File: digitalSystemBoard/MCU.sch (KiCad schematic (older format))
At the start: 33 parts, among them J1 USB-B, SW9 ButtonFirst, U10 74HC165, U11 74HC595, U6 ATmega32U4-AU, U7 ICSP, U8 74HC165, U9 74HC595, Y0 16MHz

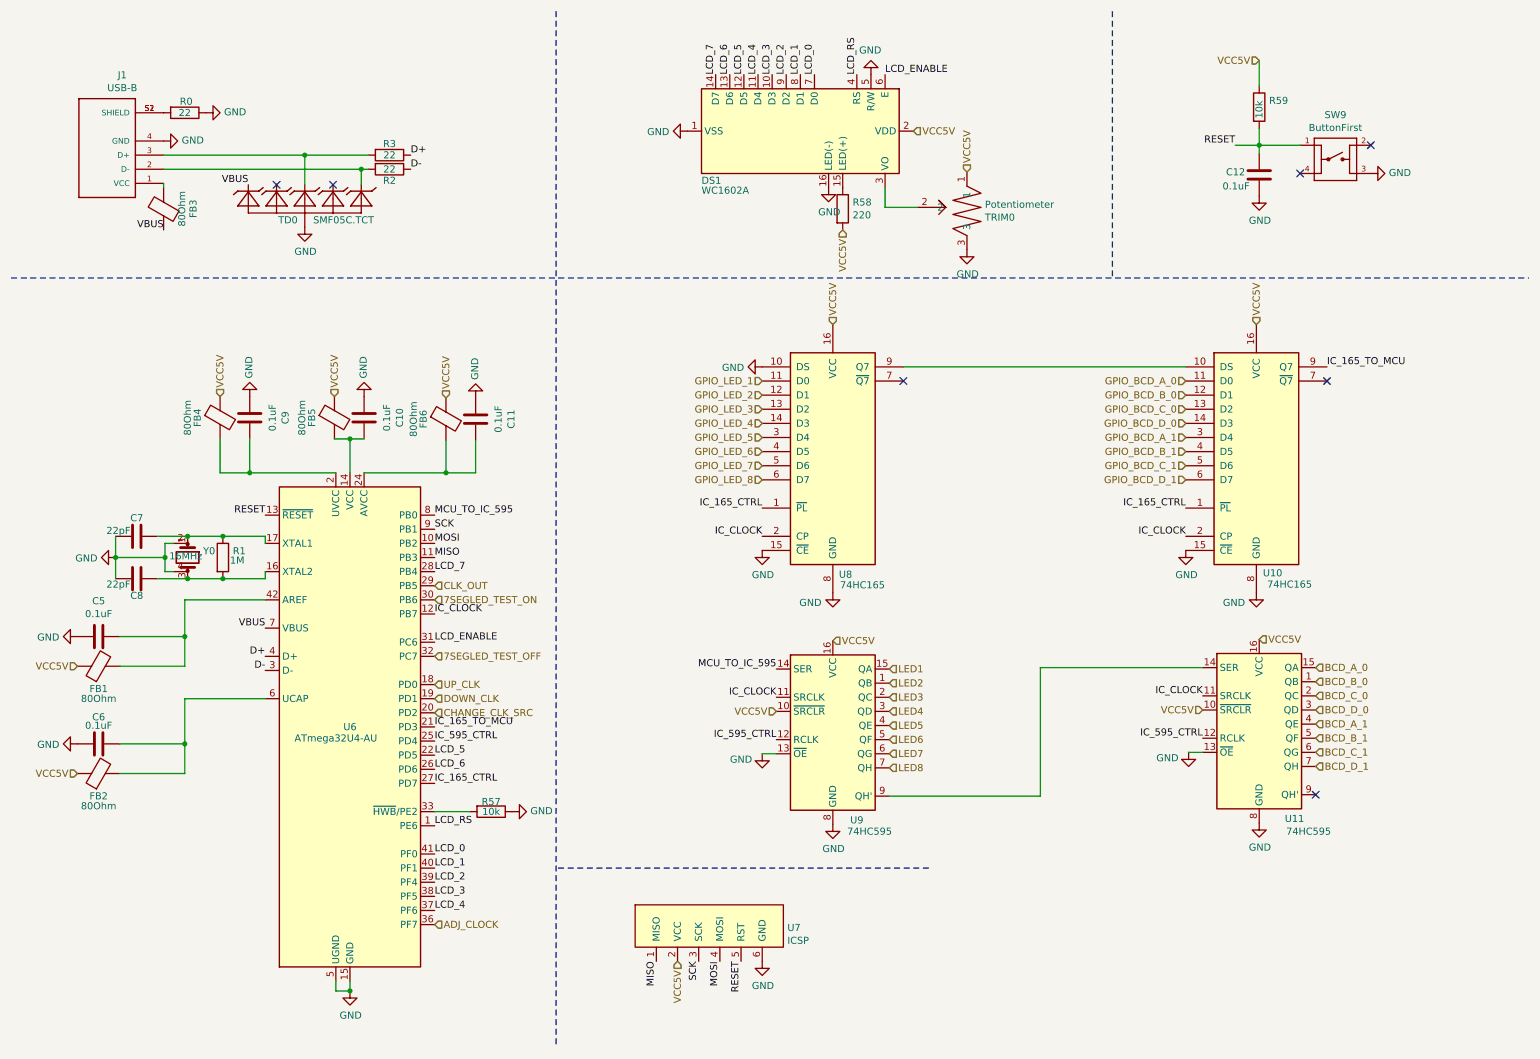
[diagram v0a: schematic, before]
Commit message: Update MCU to ATmega64A
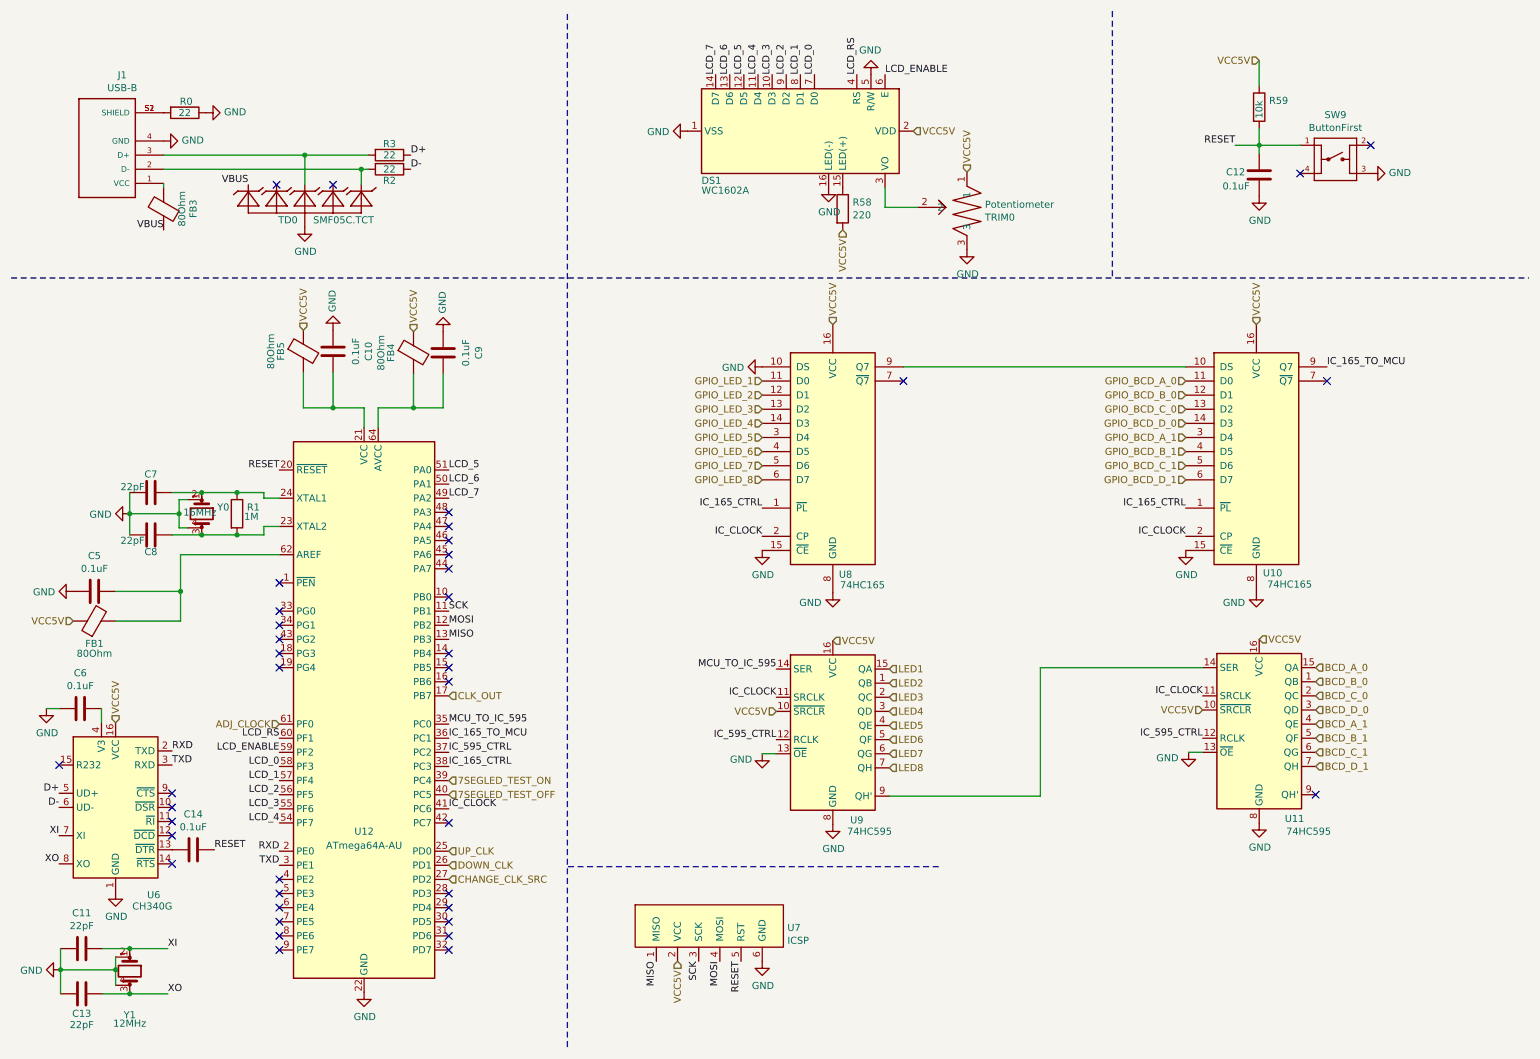
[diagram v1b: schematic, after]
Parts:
- removed FB2, FB6: 80Ohm, digitalSystemBoard:FerriteBead, symbol Device:Ferrite_Bead
- removed R57: 10k, Resistor_SMD:R_0603_1608Metric, symbol Device:R
- removed U6: ATmega32U4-AU, Package_QFP:TQFP-44_10x10mm_P0.8mm, symbol MCU_Microchip_ATmega:ATmega32U4-AU
- added C13: 22pF, Capacitor_SMD:C_0603_1608Metric, symbol Device:C
- added C14: 0.1uF, Capacitor_SMD:C_0603_1608Metric, symbol Device:C
- added U12: ATmega64A-AU, Package_QFP:TQFP-64_14x14mm_P0.8mm, symbol MCU_Microchip_ATmega:ATmega64A-AU
- added U6: CH340G, Package_SO:SOIC-16_3.9x9.9mm_P1.27mm, symbol Interface_USB:CH340G
- added Y1: 12MHz, Crystal:Crystal_SMD_Abracon_ABM8G-4Pin_3.2x2.5mm, symbol digitalSystemBoard:Resonator
- C11: value 0.1uF -> 22pF; LCSC C14663 -> C105620
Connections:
- net 7SEGLED_TEST_OFF: now also U12.40 (PC5)
- net 7SEGLED_TEST_ON: now also U12.39 (PC4)
- net ADJ_CLOCK: now also U12.61 (PF0)
- net CHANGE_CLK_SRC: now also U12.27 (PD2)
- net CLK_OUT: now also U12.17 (PB7)
- net D+: now also U6.5 (UD+)
- net D-: now also U6.6 (UD-)
- net DOWN_CLK: now also U12.26 (PD1)
- net GND: now also C13.2, U12.22 (GND), U12.53 (GND), U12.63 (GND), U6.1 (GND), Y1.2 (GND), Y1.4 (GND)
- net IC_165_CTRL: now also U12.38 (PC3)
- net IC_165_TO_MCU: now also U12.36 (PC1)
- net IC_595_CTRL: now also U12.37 (PC2)
- net IC_CLOCK: now also U12.41 (PC6)
- net LCD_0: now also U12.58 (PF3)
- net LCD_1: now also U12.57 (PF4)
- net LCD_2: now also U12.56 (PF5)
- net LCD_3: now also U12.55 (PF6)
- net LCD_4: now also U12.54 (PF7)
- net LCD_5: now also U12.51 (PA0)
- net LCD_6: now also U12.50 (PA1)
- net LCD_7: now also U12.49 (PA2)
- net LCD_ENABLE: now also U12.59 (PF2)
- net LCD_RS: now also U12.60 (PF1)
- net MCU_TO_IC_595: now also U12.35 (PC0)
- net MISO: now also U12.13 (PB3)
- net MOSI: now also U12.12 (PB2)
- net RESET: now also C14.1, U12.20 (~RESET)
- net SCK: now also U12.11 (PB1)
- net UP_CLK: now also U12.25 (PD0)
- net VCC5V: now also U6.16 (VCC)
- net at C10.1, FB5.2: now also U12.21 (VCC), U12.52 (VCC)
- net at C8.1, R1.2, Y0.3: now also U12.23 (XTAL2)
- net at C7.1, R1.1, Y0.1: now also U12.24 (XTAL1)
- net at C9.1, FB4.2: now also U12.64 (AVCC)
- net XI: now reaches C11.1
- net XI: now also U6.7 (XI), Y1.1
- net at C5.1, FB1.2: now also U12.62 (AREF)
- net at C6.1: now also U6.4 (V3)
- new net: C14.2, U6.13 (~DTR)
- new net RXD: U12.2 (PE0), U6.2 (TXD)
- new net TXD: U12.3 (PE1), U6.3 (RXD)
- new net XO: C13.1, U6.8 (XO), Y1.3
- no-connect marks 7 -> 40
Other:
- moved on the sheet: C10, C5, C7, C8, C9, FB1, FB4, FB5, R1, Y0

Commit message: Update LED footprint
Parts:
- C11, C13, C7, C8: LCSC C105620 -> C1653
- U12: LCSC (none) -> C9435
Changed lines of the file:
@@
 F 2 "Capacitor_SMD:C_0603_1608Metric" H 1498 4030 50  0001 C CNN
 F 3 "~" H 1460 4180 50  0001 C CNN
-F 4 "C105620" H 1460 4180 50  0001 C CNN "LCSC"
+F 4 "C1653" H 1460 4180 50  0001 C CNN "LCSC"
 	1    1460 4180
 	0    1    1    0
@@
 F 2 "Capacitor_SMD:C_0603_1608Metric" H 1498 3730 50  0001 C CNN
 F 3 "~" H 1460 3880 50  0001 C CNN
-F 4 "C105620" H 1460 3880 50  0001 C CNN "LCSC"
+F 4 "C1653" H 1460 3880 50  0001 C CNN "LCSC"
 	1    1460 3880
 	0    1    1    0
@@
 F 2 "Capacitor_SMD:C_0603_1608Metric" H 1008 6960 50  0001 C CNN
 F 3 "~" H 970 7110 50  0001 C CNN
-F 4 "C105620" V 970 7110 50  0001 C CNN "LCSC"
+F 4 "C1653" V 970 7110 50  0001 C CNN "LCSC"
 	1    970  7110
 	0    1    -1   0
@@
 F 2 "Capacitor_SMD:C_0603_1608Metric" H 1008 7280 50  0001 C CNN
 F 3 "~" H 970 7430 50  0001 C CNN
-F 4 "C105620" V 970 7430 50  0001 C CNN "LCSC"
+F 4 "C1653" V 970 7430 50  0001 C CNN "LCSC"
 	1    970  7430
 	0    1    1    0
@@
 F 2 "Package_QFP:TQFP-64_14x14mm_P0.8mm" H 2970 5420 50  0001 C CIN
 F 3 "http://ww1.microchip.com/downloads/en/DeviceDoc/atmel-8160-8-bit-avr-microcontroller-atmega64a-datasheet.pdf" H 2970 5420 50  0001 C CNN
+F 4 "C9435" H 2970 5420 50  0001 C CNN "LCSC"
 	1    2970 5420
 	1    0    0    -1
